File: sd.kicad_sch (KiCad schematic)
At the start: 19 parts, among them J7 112L-TDA0, J8 ST50S017VCAR1800, U6 GL3224-ONY, Y3 12MHz

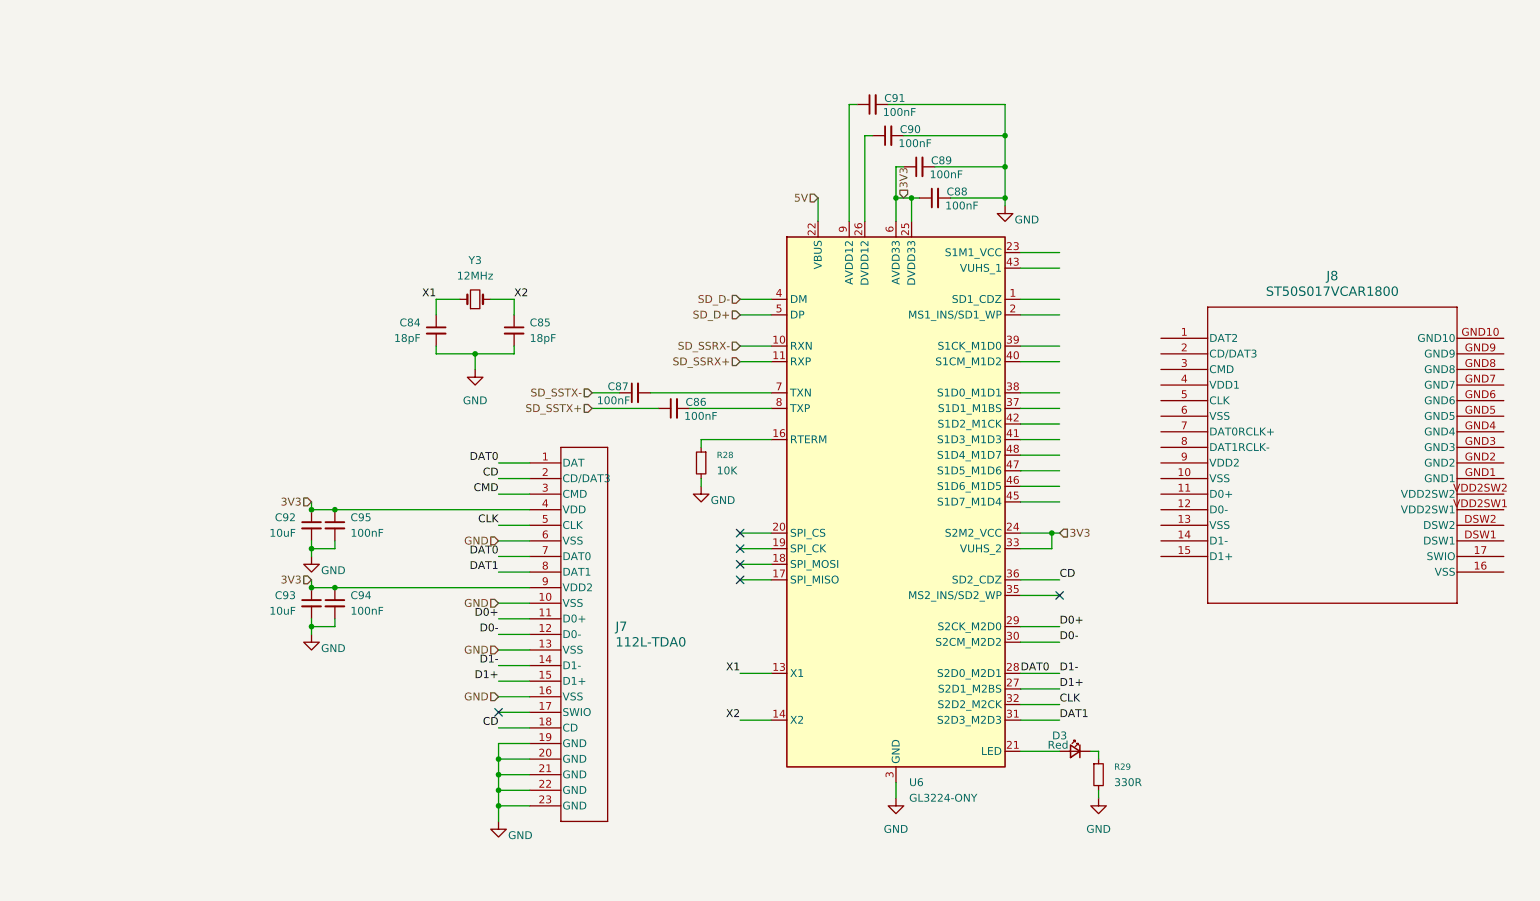
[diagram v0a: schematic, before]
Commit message: Add files via upload
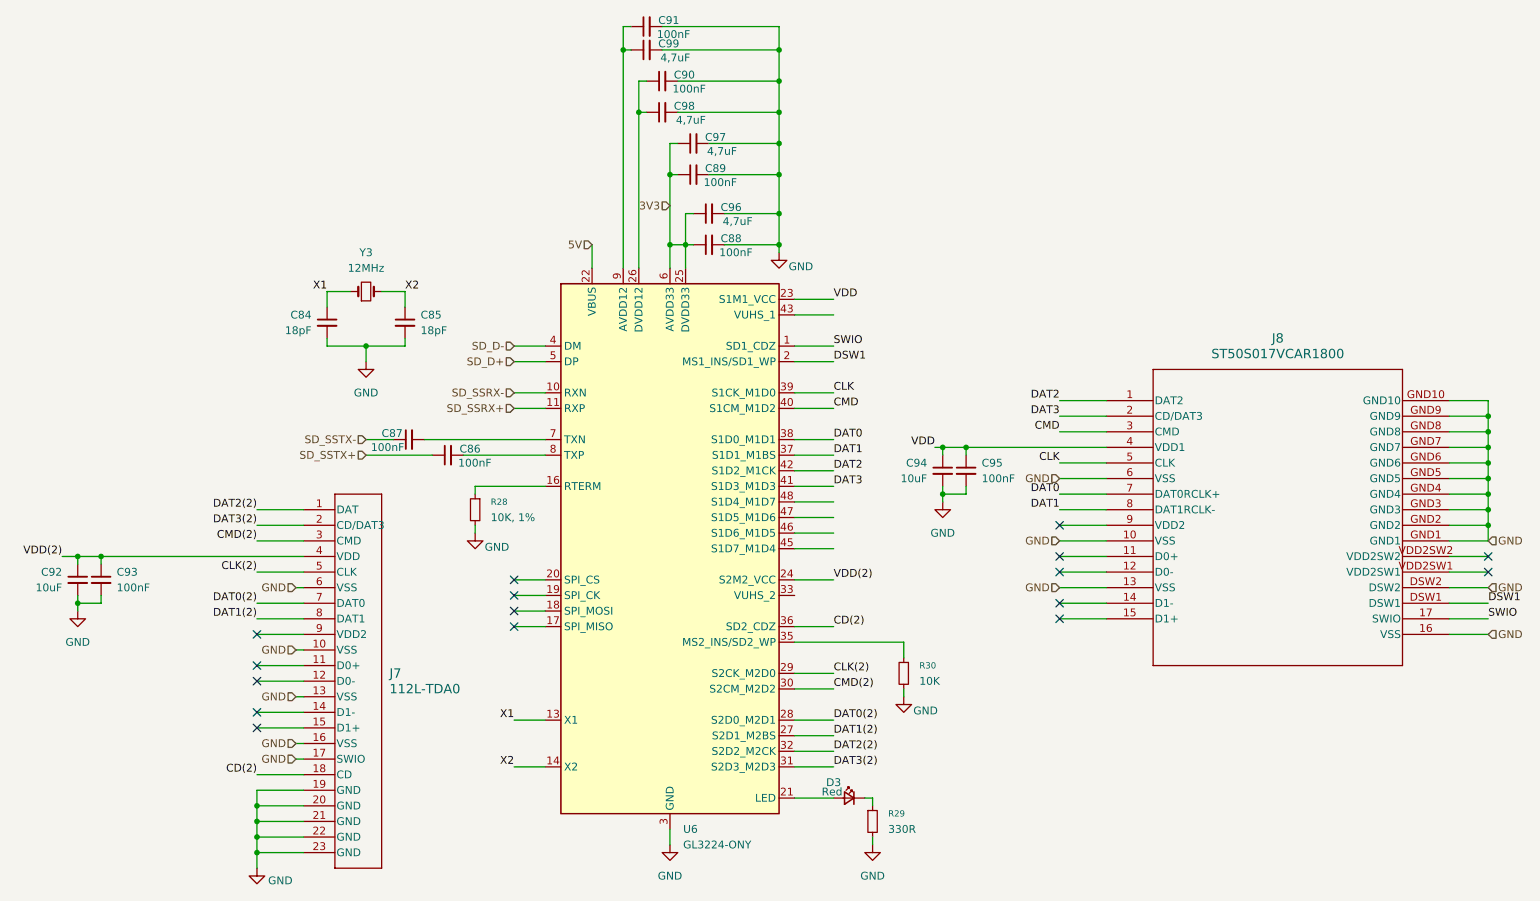
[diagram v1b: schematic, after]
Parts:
- added C96, C97, C98, C99: 4,7uF, symbol Device:C_Small
- added R30: 10K, symbol Device:R_Small
- C93: value 10uF -> 100nF
- C94: value 100nF -> 10uF
- R28: value 10K -> 10K, 1%
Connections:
- net 3V3: now also C96.1, C97.1; no longer C92.1, C93.1, C94.1, C95.1, J7.4 (VDD), J7.9 (VDD2), U6.24 (S2M2_VCC), U6.33 (VUHS_2)
- net CLK: now also J8.5 (CLK), U6.39 (S1CK_M1D0); no longer J7.5 (CLK), U6.32 (S2D2_M2CK)
- net CMD: now also J8.3 (CMD), U6.40 (S1CM_M1D2); no longer J7.3 (CMD)
- net DAT1: now also J8.8 (DAT1RCLK-), U6.37 (S1D1_M1BS); no longer J7.8 (DAT1), U6.31 (S2D3_M2D3)
- net GND: now also J7.17 (SWIO), J8.10 (VSS), J8.13 (VSS), J8.16 (VSS), J8.6 (VSS), J8.DSW2, J8.GND1, J8.GND10, J8.GND2, J8.GND3, J8.GND4, J8.GND5, J8.GND6, J8.GND7, J8.GND8, J8.GND9, C96.2, C97.2, C98.2, C99.2, R30.2
- net SWIO: now reaches U6.1 (SD1_CDZ)
- net SWIO: now also J8.17 (SWIO)
- net DSW1: now reaches U6.2 (MS1_INS/SD1_WP)
- net DSW1: now also J8.DSW1
- net VDD: now reaches U6.23 (S1M1_VCC)
- net VDD: now also C94.1, C95.1, J8.4 (VDD1)
- net at C90.1, U6.26 (DVDD12): now also C98.1
- net at U6.35 (MS2_INS/SD2_WP): now also R30.1
- net DAT0: now reaches U6.38 (S1D0_M1D1)
- net DAT0: now also J8.7 (DAT0RCLK+)
- net DAT3: now reaches U6.41 (S1D3_M1D3)
- net DAT3: now also J8.2 (CD/DAT3)
- net DAT2: now reaches U6.42 (S1D2_M1CK)
- net DAT2: now also J8.1 (DAT2)
- net at C91.1, U6.9 (AVDD12): now also C99.1
- net CD renamed CD(2)
- net CD(2): no longer J7.2 (CD/DAT3)
- net D0+: no longer names the net of J7.11 (D0+)
- net D0+: no longer U6.29 (S2CK_M2D0)
- net D0-: no longer names the net of J7.12 (D0-)
- net D0-: no longer U6.30 (S2CM_M2D2)
- net D1+: no longer names the net of J7.15 (D1+)
- net D1+: no longer U6.27 (S2D1_M2BS)
- net D1- renamed DAT0(2)
- net DAT0(2): no longer J7.1 (DAT), J7.14 (D1-)
- new net CLK(2): J7.5 (CLK), U6.29 (S2CK_M2D0)
- new net CMD(2): J7.3 (CMD), U6.30 (S2CM_M2D2)
- new net DAT1(2): J7.8 (DAT1), U6.27 (S2D1_M2BS)
- new net DAT2(2): J7.1 (DAT), U6.32 (S2D2_M2CK)
- new net DAT3(2): J7.2 (CD/DAT3), U6.31 (S2D3_M2D3)
- new net VDD(2): C92.1, C93.1, J7.4 (VDD), U6.24 (S2M2_VCC)
- no-connect marks 6 -> 16
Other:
- moved on the sheet: C84, C85, C86, C87, C88, C89, C90, C91, D3, J7, J8, R28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

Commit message: Add files via upload
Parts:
- C84, C85, C86, C87, C88, C89, C90, C91, C93, C95: footprint (none) -> Capacitor_SMD:C_0603_1608Metric
- C92, C94, C96, C97, C98, C99: footprint (none) -> Capacitor_SMD:C_1206_3216Metric
- D3: footprint (none) -> LED_SMD:LED_0603_1608Metric
- R28, R29, R30: footprint (none) -> Resistor_SMD:R_0603_1608Metric
- Y3: footprint (none) -> Crystal:Crystal_SMD_3225-4Pin_3.2x2.5mm
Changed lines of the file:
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@@
 			)
 		)
-		(property "Footprint" ""
+		(property "Footprint" "Capacitor_SMD:C_0603_1608Metric"
 			(at 85.725 90.17 0)
 			(hide yes)
@@
 			)
 		)
-		(property "Footprint" ""
+		(property "Footprint" "Capacitor_SMD:C_1206_3216Metric"
 			(at 166.37 92.71 0)
 			(hide yes)
@@
 			)
 		)
-		(property "Footprint" ""
+		(property "Footprint" "Resistor_SMD:R_0603_1608Metric"
 			(at 154.94 149.86 0)
 			(hide yes)
@@
 			)
 		)
-		(property "Footprint" ""
+		(property "Footprint" "Capacitor_SMD:C_0603_1608Metric"
 			(at 170.18 92.71 0)
 			(hide yes)
@@
 			)
 		)
-		(property "Footprint" ""
+		(property "Footprint" "Capacitor_SMD:C_0603_1608Metric"
 			(at 128.27 55.88 0)
 			(hide yes)
@@
 			)
 		)
-		(property "Footprint" ""
+		(property "Footprint" "Capacitor_SMD:C_0603_1608Metric"
 			(at 79.375 87.63 0)
 			(hide yes)
@@
 			)
 		)
-		(property "Footprint" ""
+		(property "Footprint" "Capacitor_SMD:C_0603_1608Metric"
 			(at 78.74 68.58 0)
 			(hide yes)
@@
 			)
 		)
-		(property "Footprint" ""
+		(property "Footprint" "Resistor_SMD:R_0603_1608Metric"
 			(at 90.17 99.06 0)
 			(hide yes)
@@
 			)
 		)
-		(property "Footprint" ""
+		(property "Footprint" "Capacitor_SMD:C_0603_1608Metric"
 			(at 66.04 68.58 0)
 			(hide yes)
@@
 			)
 		)
-		(property "Footprint" ""
+		(property "Footprint" "Capacitor_SMD:C_1206_3216Metric"
 			(at 125.73 39.37 0)
 			(hide yes)
@@
 			)
 		)
-		(property "Footprint" ""
+		(property "Footprint" "Capacitor_SMD:C_1206_3216Metric"
 			(at 118.11 24.13 0)
 			(hide yes)
@@
 			)
 		)
-		(property "Footprint" ""
+		(property "Footprint" "Capacitor_SMD:C_0603_1608Metric"
 			(at 29.21 110.49 0)
 			(hide yes)
@@
 			)
 		)
-		(property "Footprint" ""
+		(property "Footprint" "Capacitor_SMD:C_1206_3216Metric"
 			(at 120.65 34.29 0)
 			(hide yes)
@@
 			)
 		)
-		(property "Footprint" ""
+		(property "Footprint" "Resistor_SMD:R_0603_1608Metric"
 			(at 160.02 125.73 0)
 			(hide yes)
@@
 			)
 		)
-		(property "Footprint" ""
+		(property "Footprint" "Capacitor_SMD:C_0603_1608Metric"
 			(at 120.65 29.21 0)
 			(hide yes)
@@
 			)
 		)
-		(property "Footprint" ""
+		(property "Footprint" "Capacitor_SMD:C_0603_1608Metric"
 			(at 118.11 20.32 0)
 			(hide yes)
@@
 			)
 		)
-		(property "Footprint" ""
+		(property "Footprint" "Crystal:Crystal_SMD_3225-4Pin_3.2x2.5mm"
 			(at 72.39 63.5 0)
 			(hide yes)
@@
 			)
 		)
-		(property "Footprint" ""
+		(property "Footprint" "LED_SMD:LED_0603_1608Metric"
 			(at 151.13 146.05 90)
 			(hide yes)
@@
 			)
 		)
-		(property "Footprint" ""
+		(property "Footprint" "Capacitor_SMD:C_1206_3216Metric"
 			(at 128.27 50.8 0)
 			(hide yes)
@@
 			)
 		)
-		(property "Footprint" ""
+		(property "Footprint" "Capacitor_SMD:C_1206_3216Metric"
 			(at 25.4 110.49 0)
 			(hide yes)
@@
 			)
 		)
-		(property "Footprint" ""
+		(property "Footprint" "Capacitor_SMD:C_0603_1608Metric"
 			(at 125.73 44.45 0)
 			(hide yes)
